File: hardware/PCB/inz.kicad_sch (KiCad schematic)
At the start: 24 parts, among them J1 Conn_01x20_Socket, J10 WCS1800, J11 INA333, J12 Micro SD Adapter, J13 Relays, J2 Conn_01x20_Socket, J3 USB_C_Receptacle_USB2.0_16P, J4 Barrel_Jack_Switch, J5 J_OLED, J6 J_SGP30, J7 J_BMP1, J8 J_BMP2, J9 J_BMP3, U1 LM2596S-ADJ, U3 USBLC6-2SC6

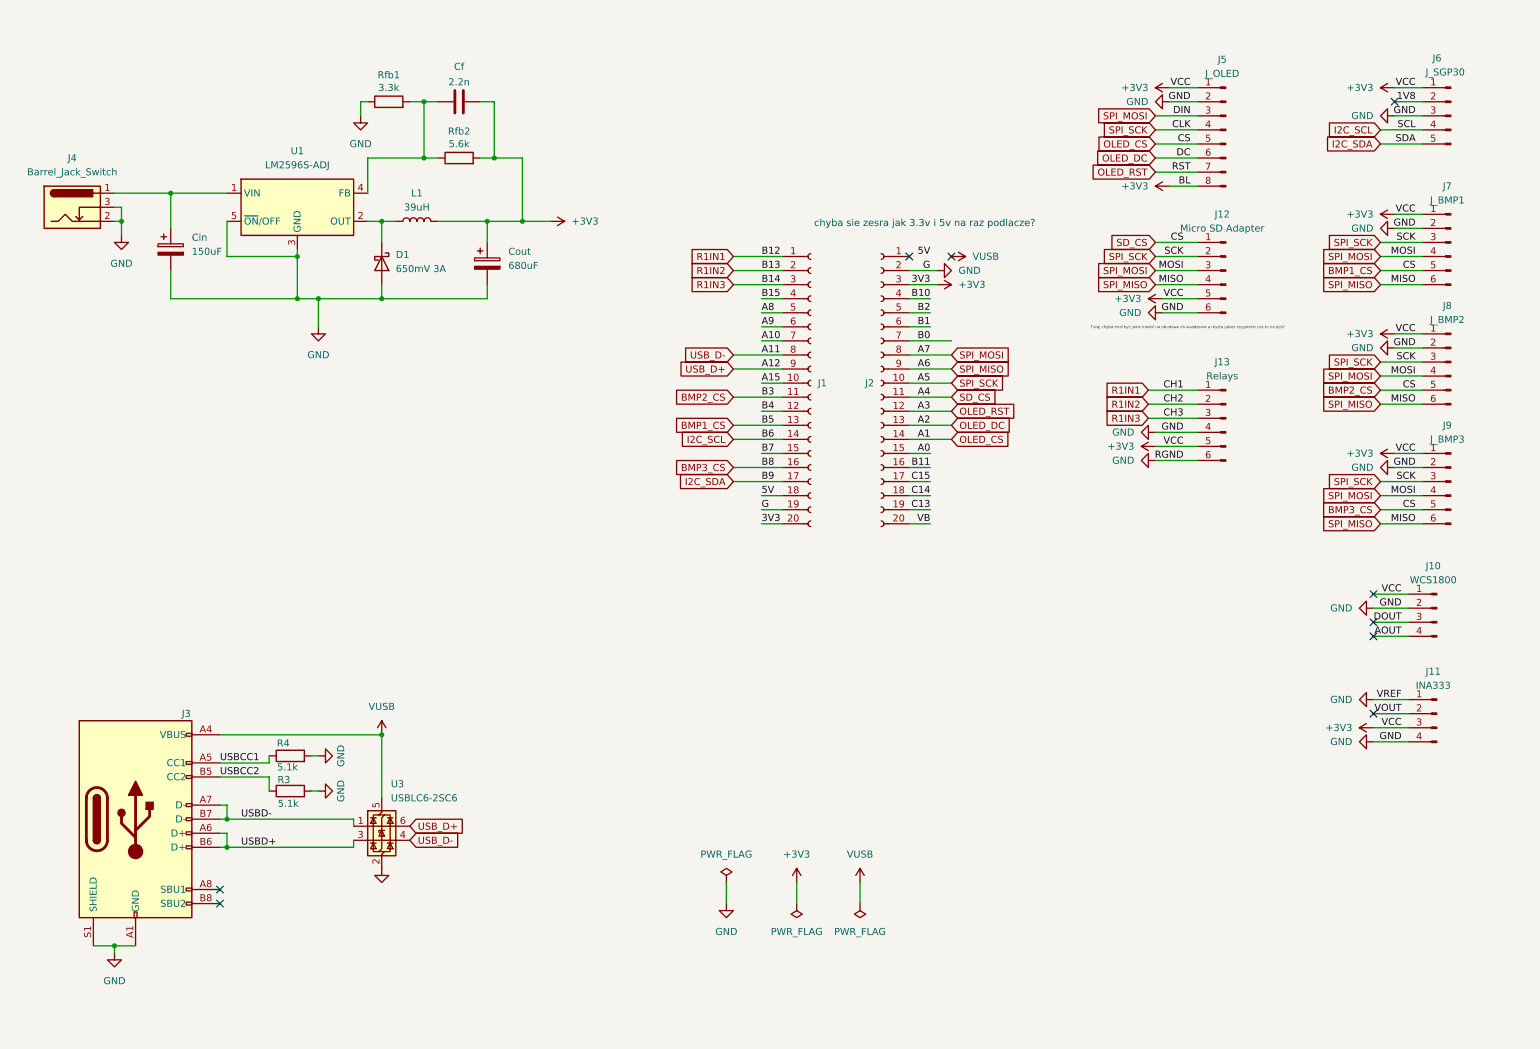
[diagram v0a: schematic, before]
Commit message: pcb
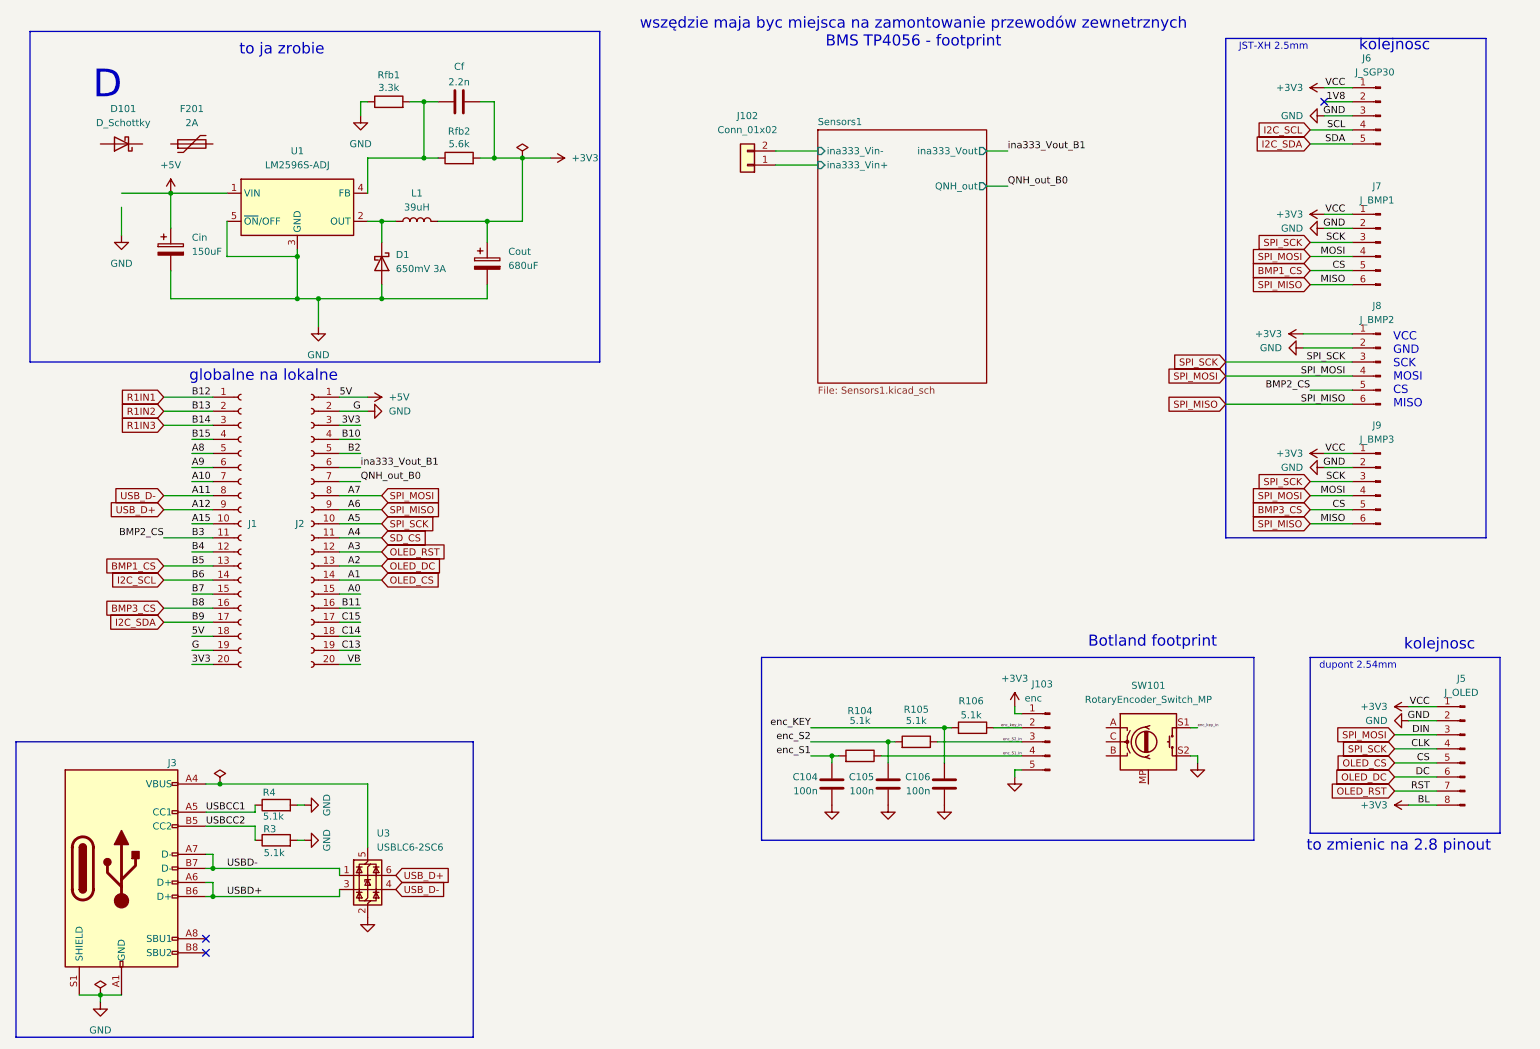
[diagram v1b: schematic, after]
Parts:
- removed J10: WCS1800, Connector_PinHeader_2.54mm:PinHeader_1x04_P2.54mm_Vertical, symbol Connector:Conn_01x04_Pin
- removed J11: INA333, Connector_PinHeader_2.54mm:PinHeader_1x04_P2.54mm_Vertical, symbol Connector:Conn_01x04_Pin
- removed J12: Micro SD Adapter, Connector_PinHeader_2.54mm:PinHeader_1x06_P2.54mm_Vertical, symbol Connector:Conn_01x06_Pin
- removed J13: Relays, Connector_PinHeader_2.54mm:PinHeader_1x06_P2.54mm_Vertical, symbol Connector:Conn_01x06_Pin
- removed J4: Barrel_Jack_Switch, Connector_BarrelJack:BarrelJack_Horizontal, symbol Connector:Barrel_Jack_Switch
- added C104, C105, C106: 100n, Capacitor_SMD:C_0805_2012Metric, symbol Device:C
- added D101: D_Schottky, Diode_SMD:D_SMA, symbol Device:D_Schottky
- added F201: 2A, Fuse:Fuseholder_Clip-5x20mm_Littelfuse_111_Inline_P20.00x5.00mm_D1.05mm_Horizontal, symbol Device:Polyfuse
- added J102: Conn_01x02, symbol Connector_Generic:Conn_01x02
- added J103: enc, Connector_PinHeader_2.54mm:PinHeader_1x05_P2.54mm_Vertical, symbol Connector:Conn_01x05_Pin
- added R104, R105, R106: 5.1k, Resistor_SMD:R_0805_2012Metric, symbol Device:R
- added SW101: RotaryEncoder_Switch_MP, symbol Device:RotaryEncoder_Switch_MP
- J5: now left out of the parts list
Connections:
- net 5V is gone; now on net +5V: J1.18 (Pin_18)
- net +3V3: now also J103.1 (Pin_1); no longer J1.20 (Pin_20), J2.3 (Pin_3)
- net BMP1_CS: no longer J1.11 (Pin_11), J2.11 (Pin_11), J8.5 (Pin_5)
- net GND: now also C104.2, C105.2, C106.2, J103.5 (Pin_5), SW101.S2
- net +5V: now reaches Cin.1, U1.1 (VIN)
- net +5V: now also J2.1 (Pin_1)
- net B0 renamed QNH_out_B0
- net B1 renamed ina333_Vout_B1
- net VUSB: no longer names the net of J3.A4 (VBUS), J3.A9 (VBUS), J3.B4 (VBUS), J3.B9 (VBUS), U3.5 (VBUS)
- new net 3V3: J1.20 (Pin_20), J2.3 (Pin_3)
- new net B3: J1.11 (Pin_11), J8.5 (Pin_5)
- new net SD_CS: J2.11 (Pin_11)
- new net Sensors1/ina333_Vin+: J102.1 (Pin_1)
- new net Sensors1/ina333_Vin-: J102.2 (Pin_2)
- new net enc_KEY: C106.1, R106.2
- new net enc_S1: C104.1, R104.2
- new net enc_S1_in: J103.4 (Pin_4), R104.1
- new net enc_S2: C105.1, R105.2
- new net enc_S2_in: J103.3 (Pin_3), R105.1
- new net enc_key_in: J103.2 (Pin_2), R106.1, SW101.S1
- no-connect marks 9 -> 3
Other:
- added sheet Sensors1 (Sensors1.kicad_sch)
- note added: "Botland footprint"
- note added: "D"
- note added: "JST-XH 2.5mm"
- note added: "VCC GND SCK MOSI CS MISO"
- note added: "dupont 2.54mm"
- note added: "globalne na lokalne"
- note added: "kolejnosc"
- note added: "to ja zrobie"
- note added: "to zmienic na 2.8 pinout"
- note added: "wszędzie maja byc miejsca na zamontowanie przewodów zewnetrznych BMS TP4056 - footprint"
- note removed: "Tutaj chyba mial byc jakis modul na obudowe do wsadzania a reszta jakies rezystorki cos to na pcb?"
- note removed: "chyba sie zesra jak 3.3v i 5v na raz podlacze?"
- moved on the sheet: J1, J2, J3, J5, J6, J7, J8, J9, R3, R4, U3
